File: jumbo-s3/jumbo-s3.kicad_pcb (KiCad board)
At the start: 2 copper layers, 40.5 x 27.3 mm, 26 parts, among them J1 UART, J2 GPIO, U1 ESP32-S3, U2 APS12808L-3OBM-BA, Y1 40MHz 10ppm

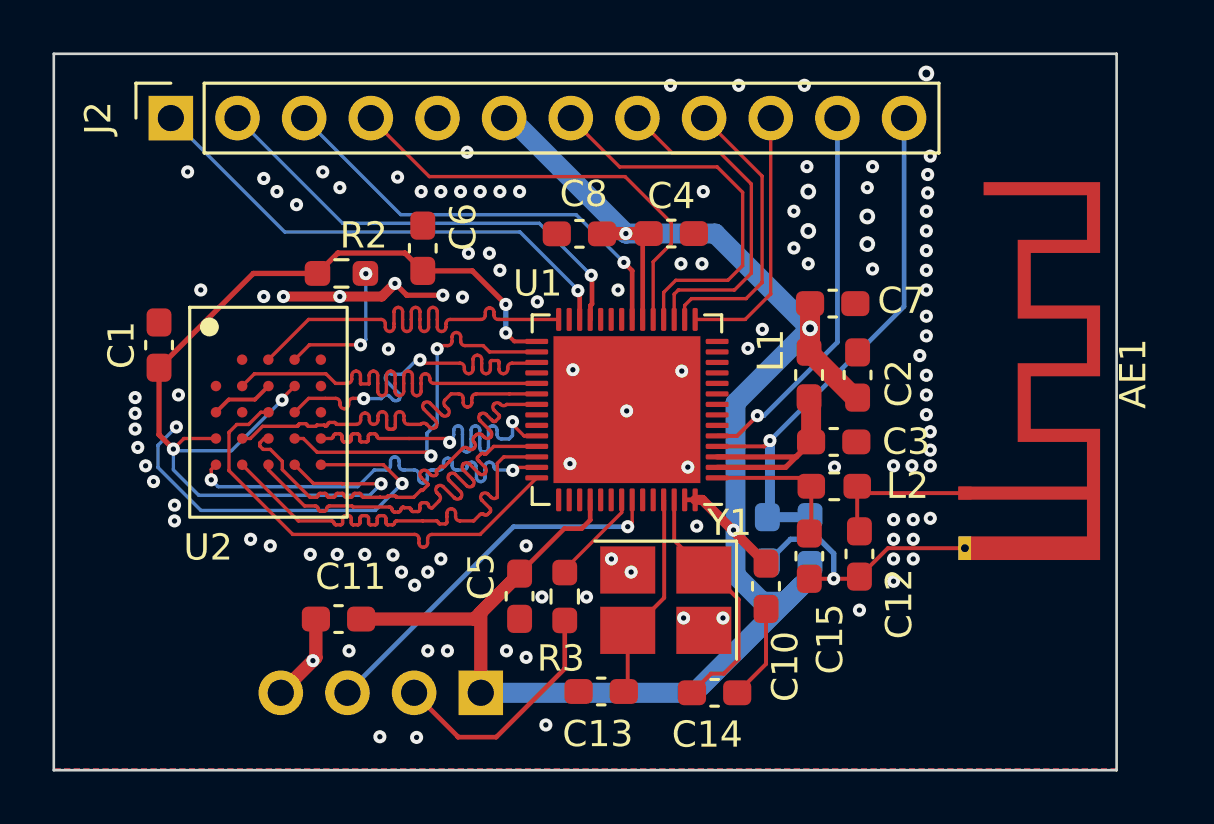
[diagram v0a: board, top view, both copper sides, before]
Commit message: Rev 2: init
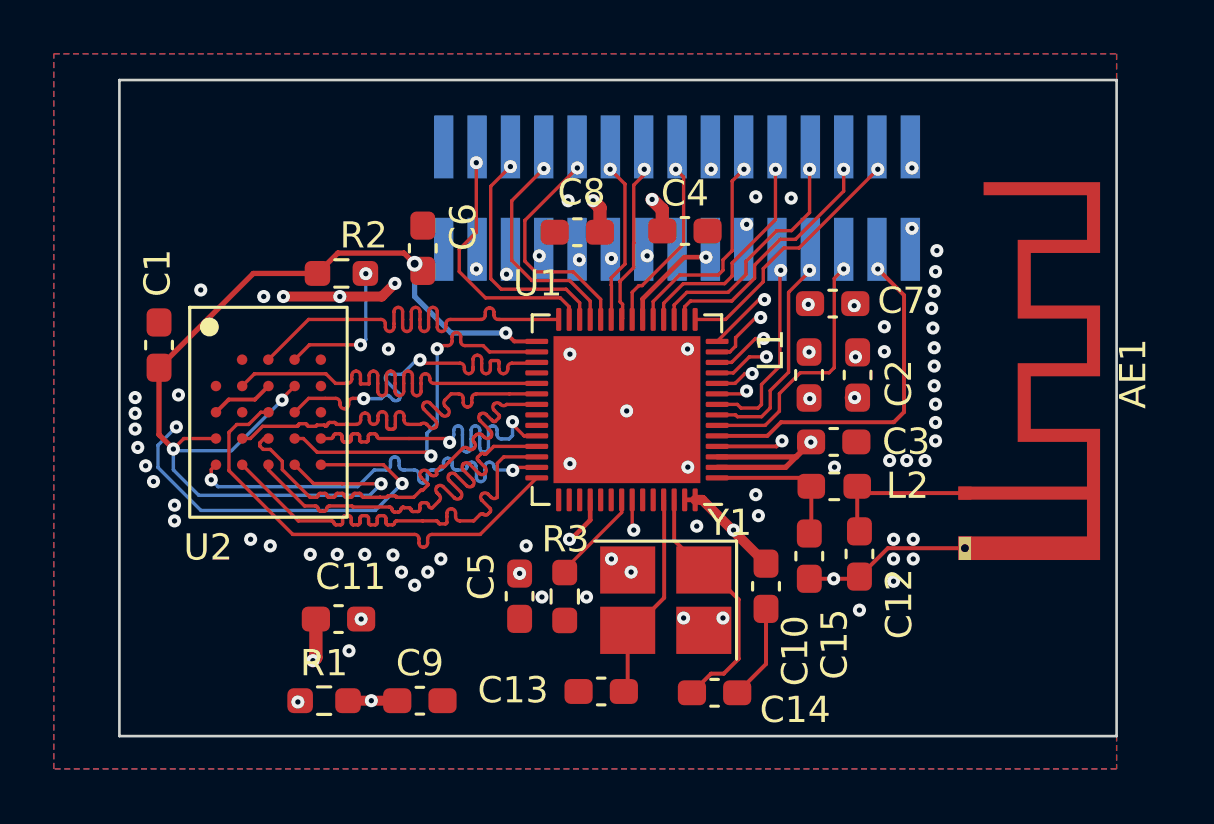
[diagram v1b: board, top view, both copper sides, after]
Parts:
- removed J2: GPIO, Connector_PinSocket_2.54mm:PinSocket_1x12_P2.54mm_Vertical
- C9, R1: moved to F.Cu
- J1: value UART -> GPIO; footprint Connector_PinHeader_2.54mm:PinHeader_1x04_P2.54mm_Vertical -> Connector_PinHeader_1.27mm:PinHeader_2x15_P1.27mm_Vertical_SMD
- moved J1 20.3 mm to (168.2, 119.5)
- moved R1 19.5 mm to (154.8, 138.7), turned to 0 degrees
- moved C9 14.6 mm to (158.4, 138.7), turned to 0 degrees
- moved C4 0.53 mm to (168.6, 120.8)
- moved C8 0.10 mm to (164.4, 120.8)
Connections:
- J1 pad 2: TxD -> +3.3V
- J1 pad 3: RxD -> GPIO0
- J1 pad 4: GND -> GPIO10
- U1 pad 10: unconnected-(U1-Pad10) -> GPIO5
- U1 pad 11: unconnected-(U1-Pad11) -> GPIO6
- U1 pad 12: unconnected-(U1-Pad12) -> GPIO7
- U1 pad 13: unconnected-(U1-Pad13) -> GPIO8
- U1 pad 14: unconnected-(U1-Pad14) -> GPIO9
- U1 pad 22: unconnected-(U1-Pad22) -> GPIO16
- U1 pad 23: unconnected-(U1-Pad23) -> GPIO17
- U1 pad 24: unconnected-(U1-Pad24) -> GPIO18
- U1 pad 27: unconnected-(U1-Pad27) -> GPIO21
- U1 pad 6: unconnected-(U1-Pad6) -> GPIO1
- U1 pad 7: unconnected-(U1-Pad7) -> GPIO2
- U1 pad 8: unconnected-(U1-Pad8) -> GPIO3
- U1 pad 9: unconnected-(U1-Pad9) -> GPIO4
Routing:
- net +3.3V: track 73.7 -> 15.2 mm, vias 3 -> 14
- net GPIO6: track 0.00 -> 14.9 mm, vias 0 -> 2
- net GPIO4: track 0.00 -> 14.6 mm, vias 0 -> 2
- net GPIO5: track 0.00 -> 14.0 mm, vias 0 -> 2
- net GPIO7: track 0.00 -> 13.2 mm, vias 0 -> 2
- net RxD: track 14.4 -> 1.18 mm
- net GPIO20: track 19.4 -> 8.98 mm
- net GPIO15: track 16.8 -> 6.73 mm
- net GPIO8: track 0.00 -> 9.79 mm, vias 0 -> 2
- net GPIO1: track 0.00 -> 9.67 mm, vias 0 -> 1
- net GPIO21: track 0.00 -> 9.65 mm, vias 0 -> 1
- net TxD: track 9.37 -> 0.00 mm
- net GPIO19: track 17.7 -> 8.34 mm
- net GPIO14: track 17.1 -> 8.02 mm, vias 0 -> 1
- net GPIO18: track 0.00 -> 8.64 mm, vias 0 -> 1
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- added copper zone on In2.Cu, net +3.3V
- added copper zone on In1.Cu, net GND
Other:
- board size 40.5 x 27.3 mm -> 38 x 25 mm
- copper layers 2 -> 4
- board text removed: "EN 0 10 11 12 13 VCC GND 14 15 19 20"
- board text removed: "GND RxD TxD 3V3"
